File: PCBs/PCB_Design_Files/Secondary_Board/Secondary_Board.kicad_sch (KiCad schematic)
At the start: 6 parts, among them J1 Conn_FFC_8pin, J2 Conn_01x08_Pin

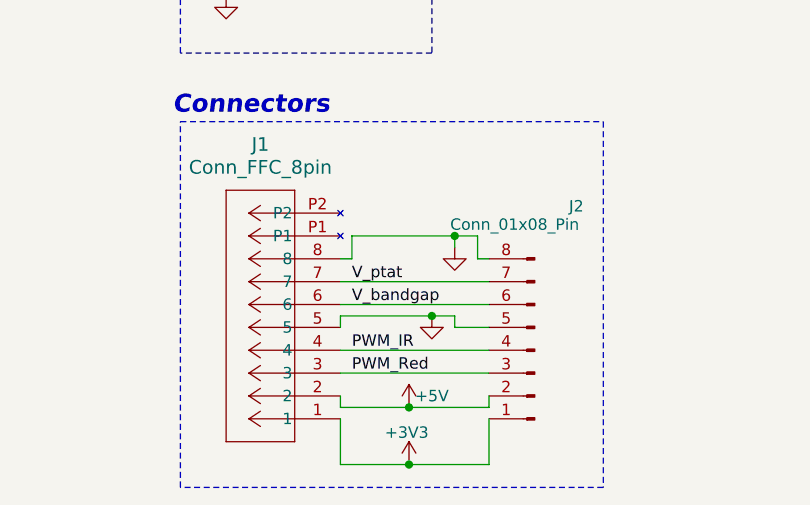
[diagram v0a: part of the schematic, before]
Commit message: updated bg_ptat
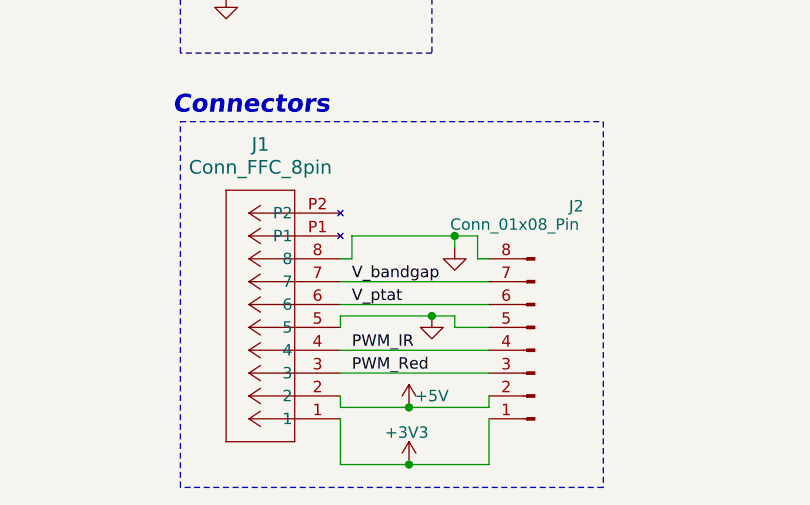
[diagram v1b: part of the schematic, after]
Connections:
- net V_bandgap: now also J1.7, J2.7 (Pin_7); no longer J1.6, J2.6 (Pin_6)
- net V_ptat: now also J1.6, J2.6 (Pin_6); no longer J1.7, J2.7 (Pin_7)
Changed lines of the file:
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@@
 		)
 	)
-	(label "V_bandgap"
+	(label "V_ptat"
 		(at 41.91 107.95 0)
 		(effects
@@
 	)
 	(label "V_bandgap"
+		(at 41.91 105.41 0)
+		(effects
+			(font
+				(size 1.27 1.27)
+			)
+			(justify left bottom)
+		)
+	)
+	(label "V_bandgap"
 		(at 238.76 52.07 0)
 		(effects
@@
 		(effects
 			(font
-				(size 1.27 1.27)
-			)
-			(justify left bottom)
-		)
-	)
-	(label "V_ptat"
-		(at 41.91 105.41 0)
-		(effects
-			(font
